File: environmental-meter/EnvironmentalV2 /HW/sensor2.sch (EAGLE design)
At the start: 16 parts

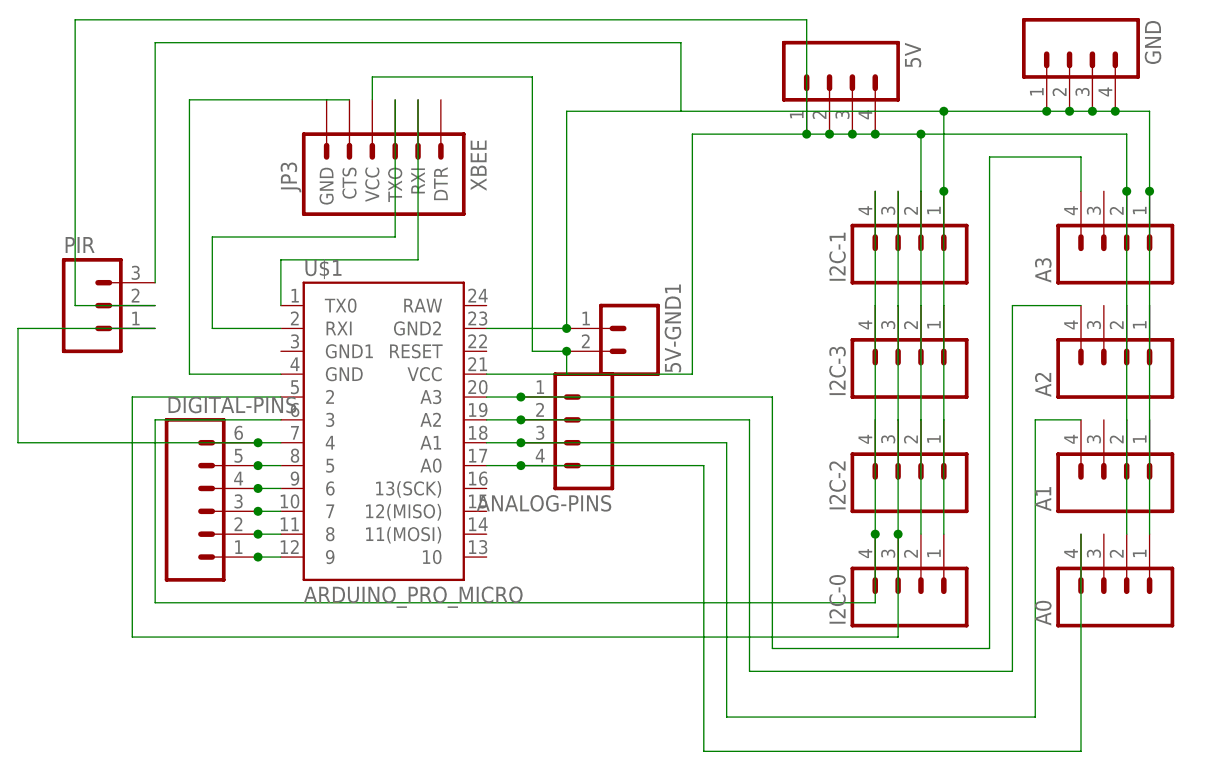
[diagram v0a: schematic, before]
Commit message: EnvironmentalV2 update version
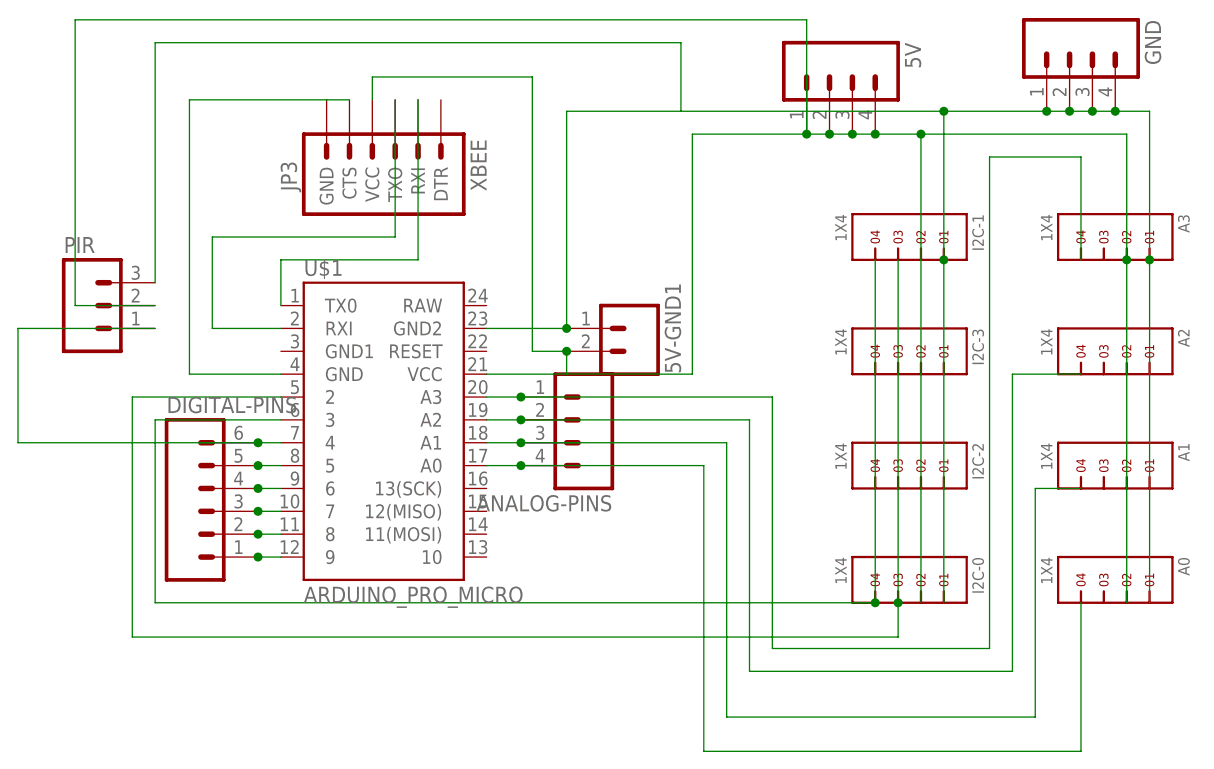
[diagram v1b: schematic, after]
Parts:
- A0, A1, A2, A3, I2C-0, I2C-1, I2C-2, I2C-3: value (none) -> 1X4; device SparkFun-Connectors:M04JST -> headers(2mm):1X4
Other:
- moved on the sheet: A0, A1, A2, A3, I2C-0, I2C-1, I2C-2, I2C-3
